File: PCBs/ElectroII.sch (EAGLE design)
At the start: 15 parts, among them J1 U.FL-R-SMT(01), U1 RFM95W-868S2

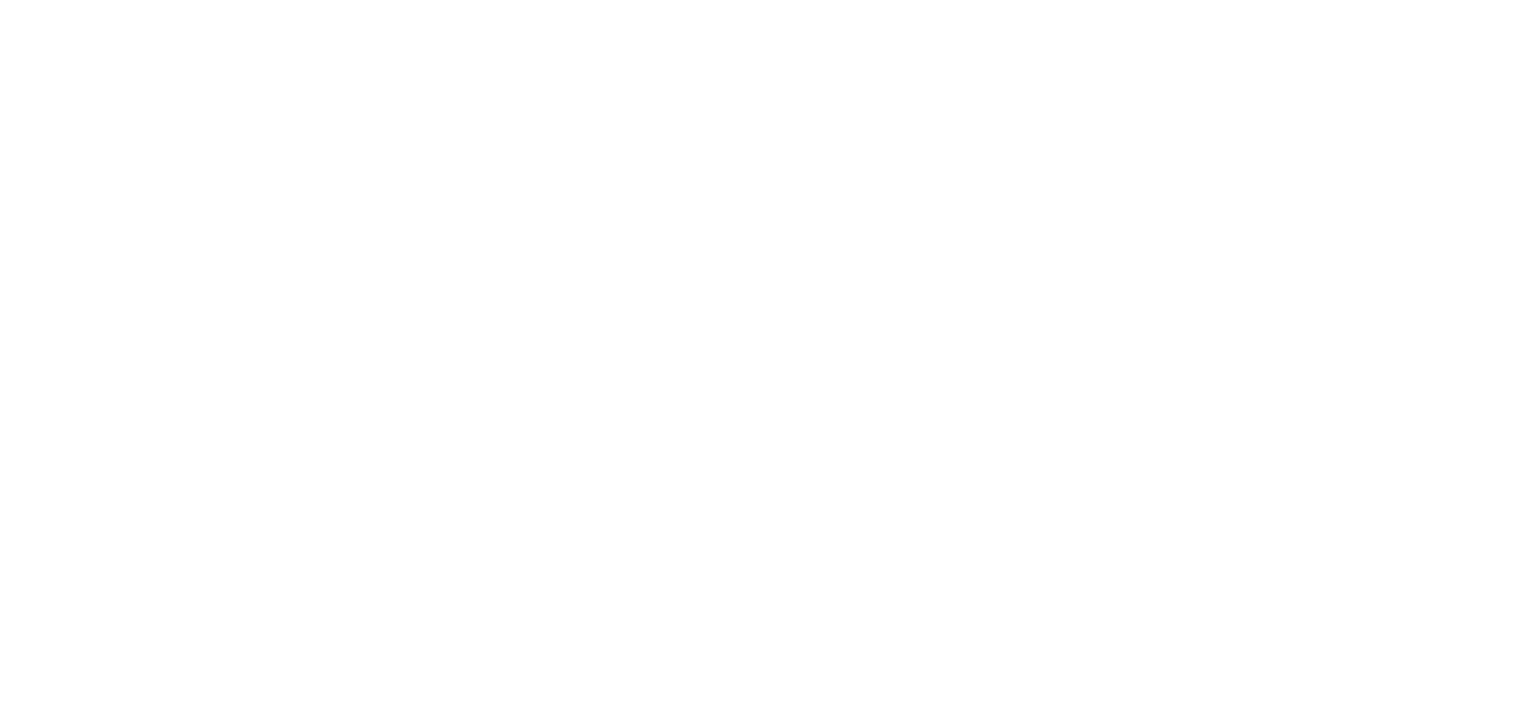
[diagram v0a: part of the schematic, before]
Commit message: Lots of progress on boost converter
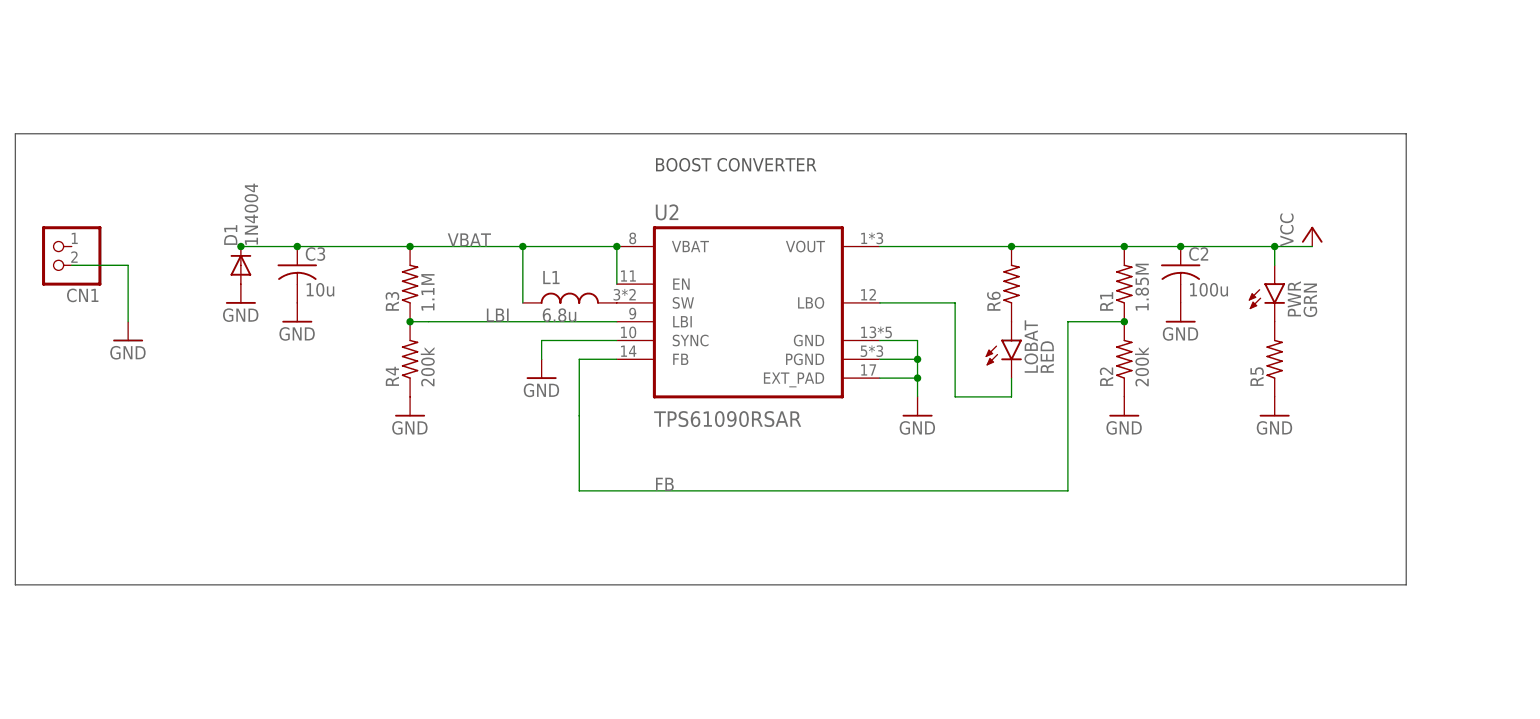
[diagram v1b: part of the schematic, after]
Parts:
- added C2: 100u, RTR Main Library:C-ALL_PACKAGESC1206
- added C3: 10u, RTR Main Library:C-ALL_PACKAGESC1206
- added CN1: (no value), adafruit:JST_2PIN-SMT-RA
- added D1: 1N4004, adafruit:1N4004
- added L1: 6.8u, RTR Main Library:L_SMD
- added LOBAT: RED, RTR Main Library:LED5MM
- added PWR: GRN, RTR Main Library:LED5MM
- added R1: 1.85M, RTR Main Library:R-ALL_PACKAGESR1206
- added R2, R4: 200k, RTR Main Library:R-ALL_PACKAGESR1206
- added R3: 1.1M, RTR Main Library:R-ALL_PACKAGESR1206
- added R5, R6: (no value), RTR Main Library:R-ALL_PACKAGESR1206
- added U2: TPS61090RSAR, TPS61090RSAR:TPS61090RSAR
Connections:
- new net FB: R1.1, R2.2, U2.FB
- new net LBI: R3.1, R4.2, U2.LBI
- new net N$1: LOBAT.A, R6.1
- new net N$2: LOBAT.C, U2.LBO
- new net N$4: L1.2, U2.SW
- new net N$5: PWR.C, R5.2
- new net VBAT: C3.1, D1.C, L1.1, R3.2, U2.EN, U2.VBAT
- net GND: now also C2.2, C3.2, CN1.1, D1.A, R2.1, R4.1, R5.1, U2.EXT_PAD, U2.GND, U2.PGND, U2.SYNC
- net VCC: now also C2.1, PWR.A, R1.2, R6.2, U2.VOUT
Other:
- note added: "BOOST CONVERTER"
